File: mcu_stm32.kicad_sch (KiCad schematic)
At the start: 23 parts, among them J1 Debug, J2 Boot_Sel, SW1 RESET, U1 STM32F103C8Tx, Y1 8mHz, Y2 32.768kHz

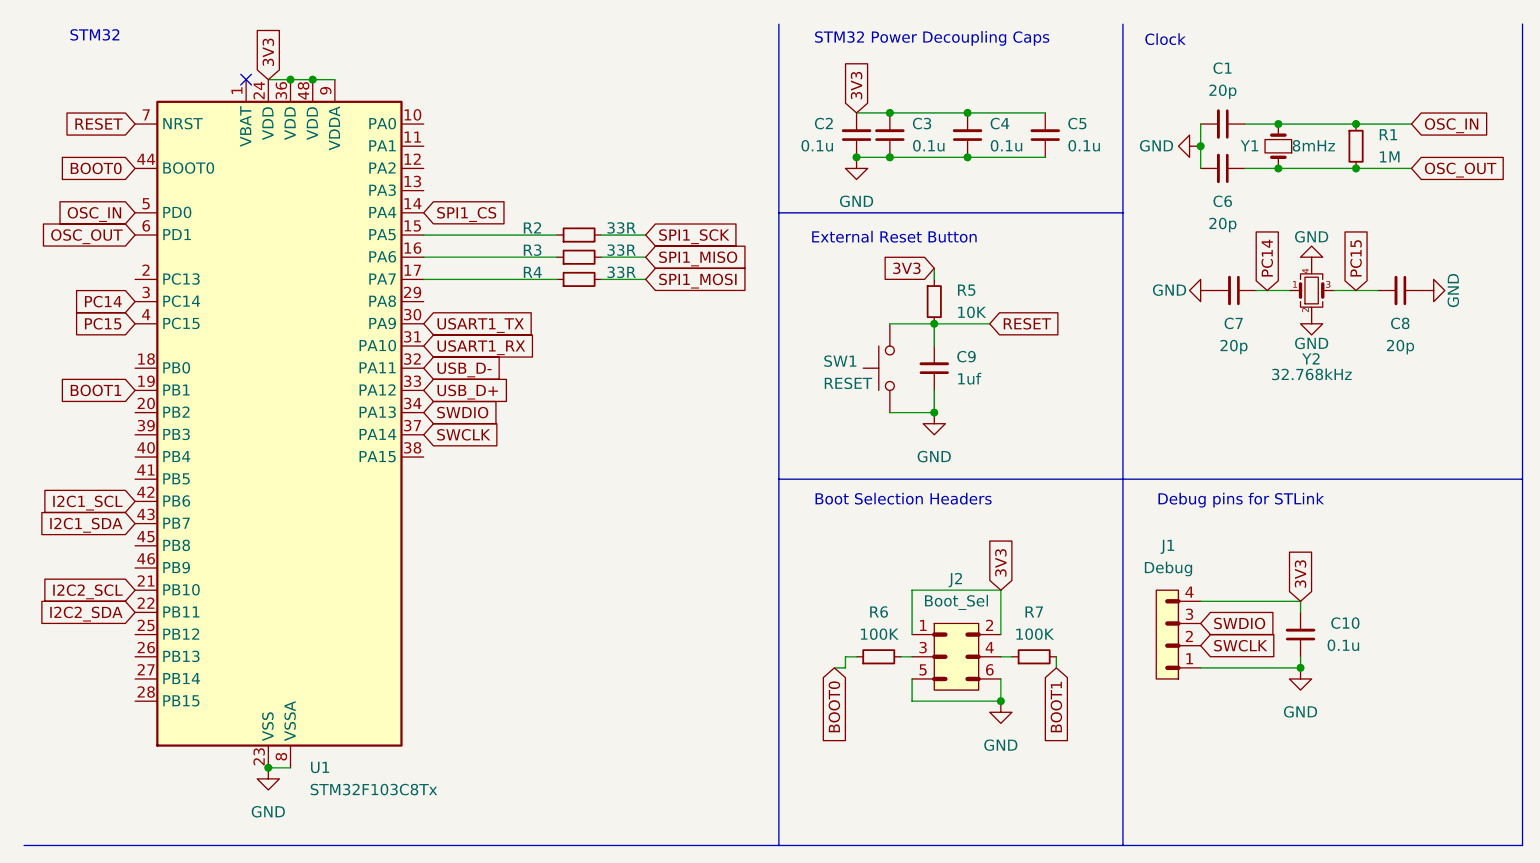
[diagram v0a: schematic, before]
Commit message: Routing
Routing ESP32 and Components
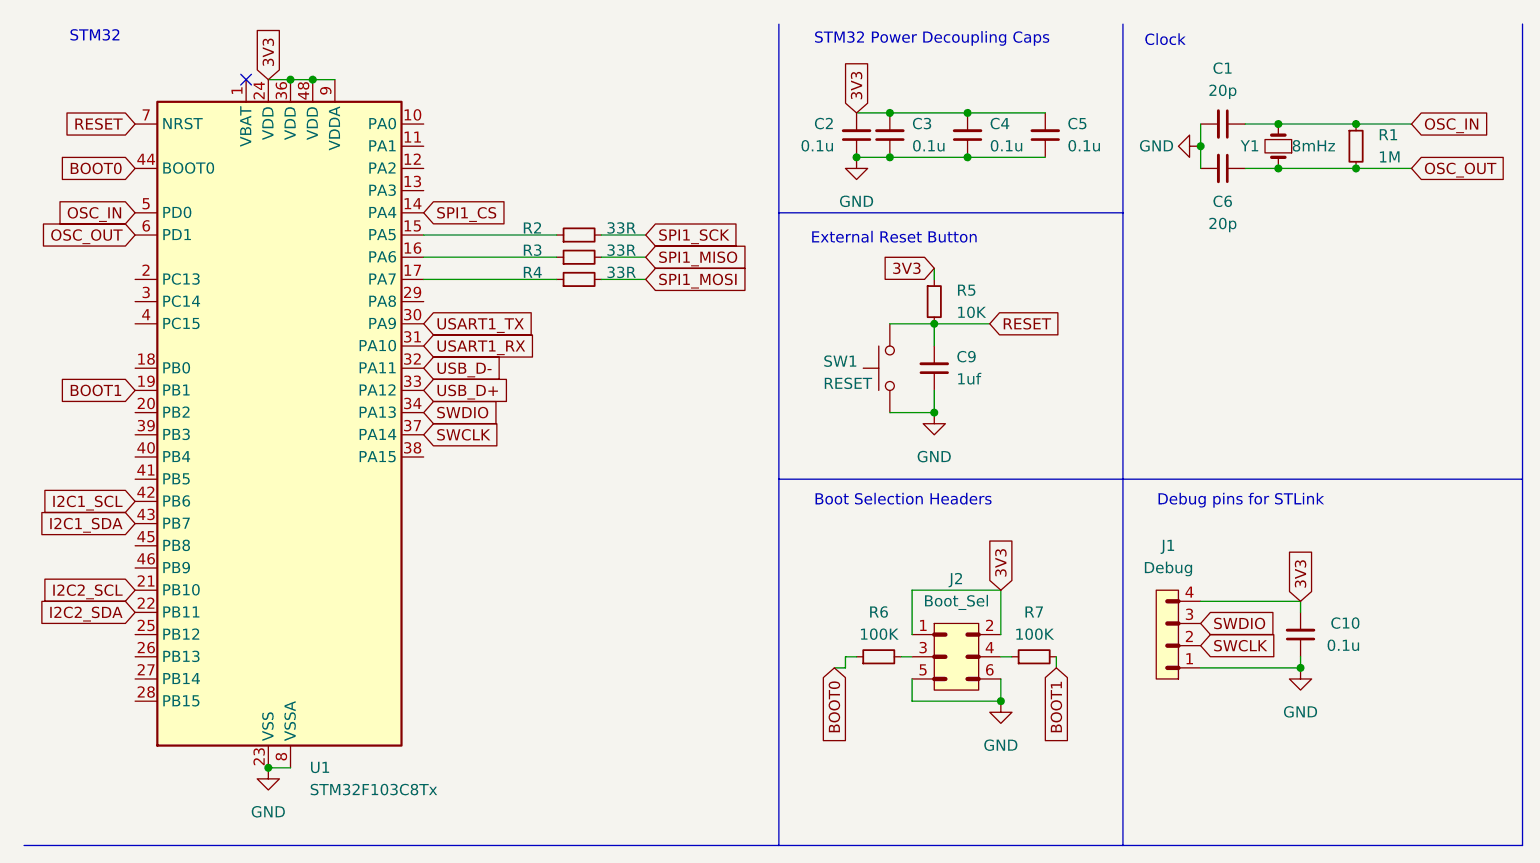
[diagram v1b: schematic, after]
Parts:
- removed C7, C8: 20p, Capacitor_SMD:C_0805_2012Metric, symbol Device:C_Small
- removed Y2: 32.768kHz, Crystal:Crystal_SMD_2016-4Pin_2.0x1.6mm, symbol Device:Crystal_GND24_Small
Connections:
- net PC14: no longer names the net of U1.3 (PC14)
- net PC15: no longer names the net of U1.4 (PC15)
